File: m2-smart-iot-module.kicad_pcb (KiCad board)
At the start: 4 copper layers, 80.2 x 22.1 mm, 198 parts, among them IC1 UPD720201K8-711-BAC-A, J1 MM8130-2600RA2, J2 2X05, J3 M.2-M+B-Pins, Q1 BSS123, SW1 PTS840_GK_SMTR_LFS, SW2 PTS840_GK_SMTR_LFS, U1 FT2232H-56Q, U10 MIC2877-5.0YFT-TR, U11 93LC56CT-IMC, U2 SST25VF512A, U3 CoralAccelerator, U4 NRF52840, U5 AP2120N-1.8TRG1, U6 AP22652W6-7, U7 TLV803EF29DBZR, U8 BME280, U9 NCP1599MNTWG, Y1 NX3225SA-24M, Y2 ABM11W-101-32.0000MHZ-T3, Y3 ABS06-32.768KHZ-9-1-T, Y4 ABM8G-12M-18-D2Y-T

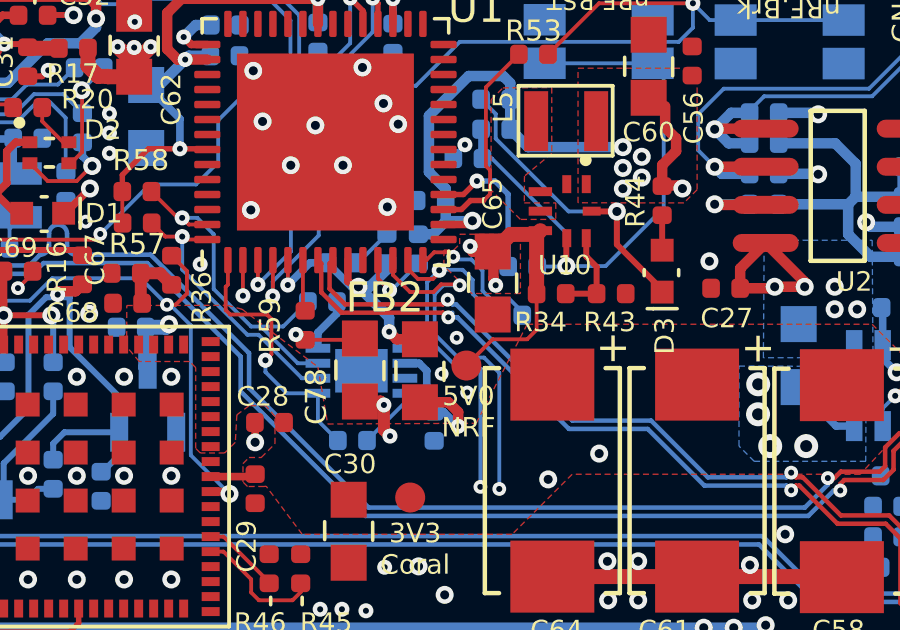
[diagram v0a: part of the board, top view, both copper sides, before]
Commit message: Bumped version
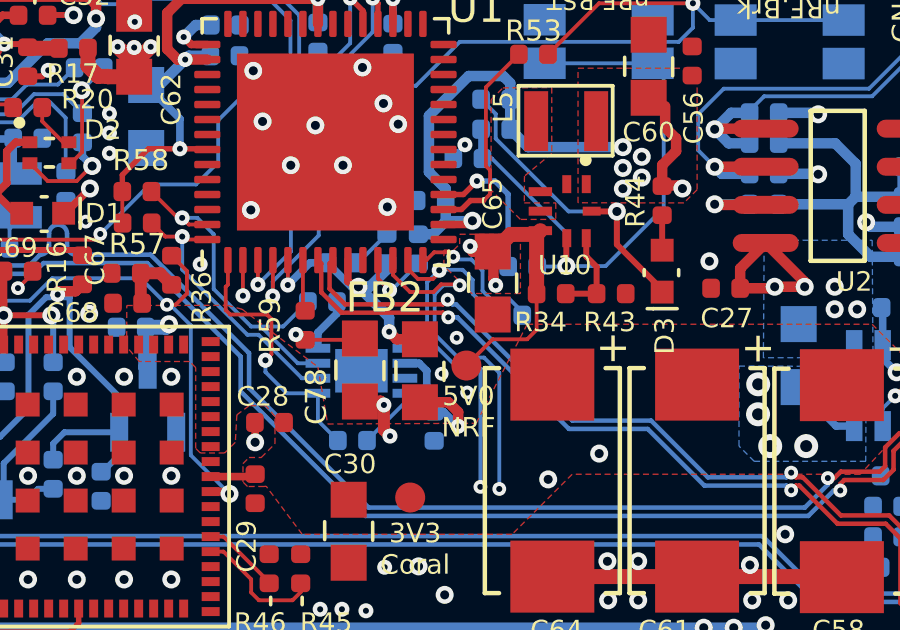
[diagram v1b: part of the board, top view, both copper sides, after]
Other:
- board text added: "rev 1.2.3"
- board text removed: "rev 1.2.1"
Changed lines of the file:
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@@
   (title_block
     (date "2022-07-11")
-    (rev "1.2.1")
+    (rev "1.2.3")
   )
   (layers
@@
     (effects (font (size 0.65 0.65) (thickness 0.15)) (justify mirror))
   )
-  (gr_text "rev 1.2.1" (at 185.928 94.05) (layer "B.Mask")
+  (gr_text "rev 1.2.3" (at 185.928 94.05) (layer "B.Mask")
     (effects (font (size 0.65 0.65) (thickness 0.15)) (justify mirror))
   )
@@
   (segment (start 172.145 108.3785) (end 172.3 108.5335) (width 0.15) (layer "B.Cu") (net 39))
   (segment (start 167.51763 106.4885) (end 169.40763 108.3785) (width 0.15) (layer "B.Cu") (net 39))
-  (segment (start 161.005 102.6135) (end 160.85 102.7685) (width 0.15) (layer "B.Cu") (net 39))
   (segment (start 169.40763 108.3785) (end 172.145 108.3785) (width 0.15) (layer "B.Cu") (net 39))
   (segment (start 161.17263 102.7685) (end 164.89263 106.4885) (width 0.15) (layer "B.Cu") (net 39))
